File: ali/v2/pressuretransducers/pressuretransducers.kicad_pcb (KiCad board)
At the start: 4 copper layers, 85 x 76 mm, 235 parts, among them J1 Conn_02x01, J10 Conn_01x02, J11 Conn_01x02, J12 Conn_01x02, J13 Conn_01x02, J14 Conn_01x02, J15 Conn_01x02, J16 Conn_01x02, J17 Conn_01x02, J18 Conn_01x02, J19 Conn_01x02, J2 Conn_01x05, J20 Conn_01x02, J21 Conn_01x02, J22 Conn_01x02, J23 Conn_01x02, J24 Conn_01x02, J25 Conn_01x02, J3 USB_C_Receptacle_USB2.0_16P, J4 Conn_01x15, J5 Conn_02x09_Counter_Clockwise, J6 Screw_Terminal_01x02, J7 Screw_Terminal_01x02, J8 Conn_01x03, J9 Vertical Ethernet, SW1 SKRPANE010, U1 STM32H563RIV6, U2 AP2112K-3.3, U3 TJA1462ATK, U4 LAN8742AI, U5 ADS131M08IRSN, U6 ADS131M08IRSN, Y1 25 MHz, Y2 8.192 MHz, Y3 25 MHz

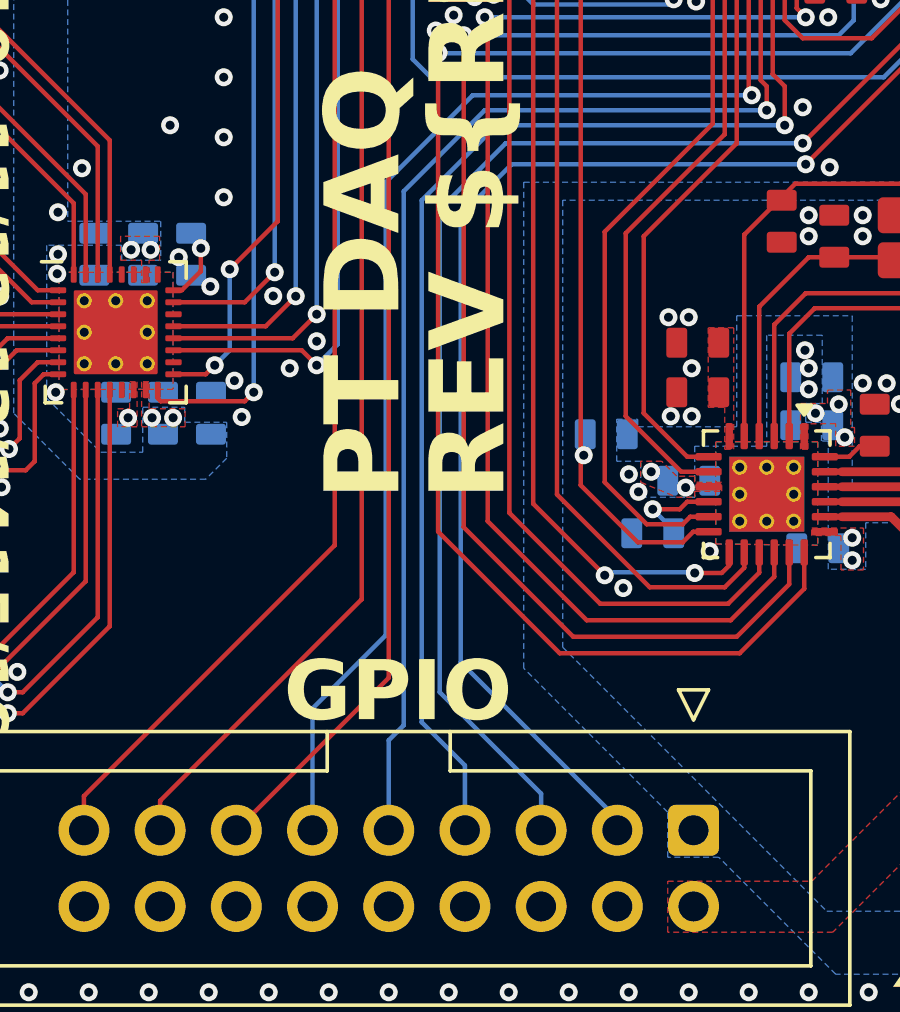
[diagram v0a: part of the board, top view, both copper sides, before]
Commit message: Minor thermocouple updates
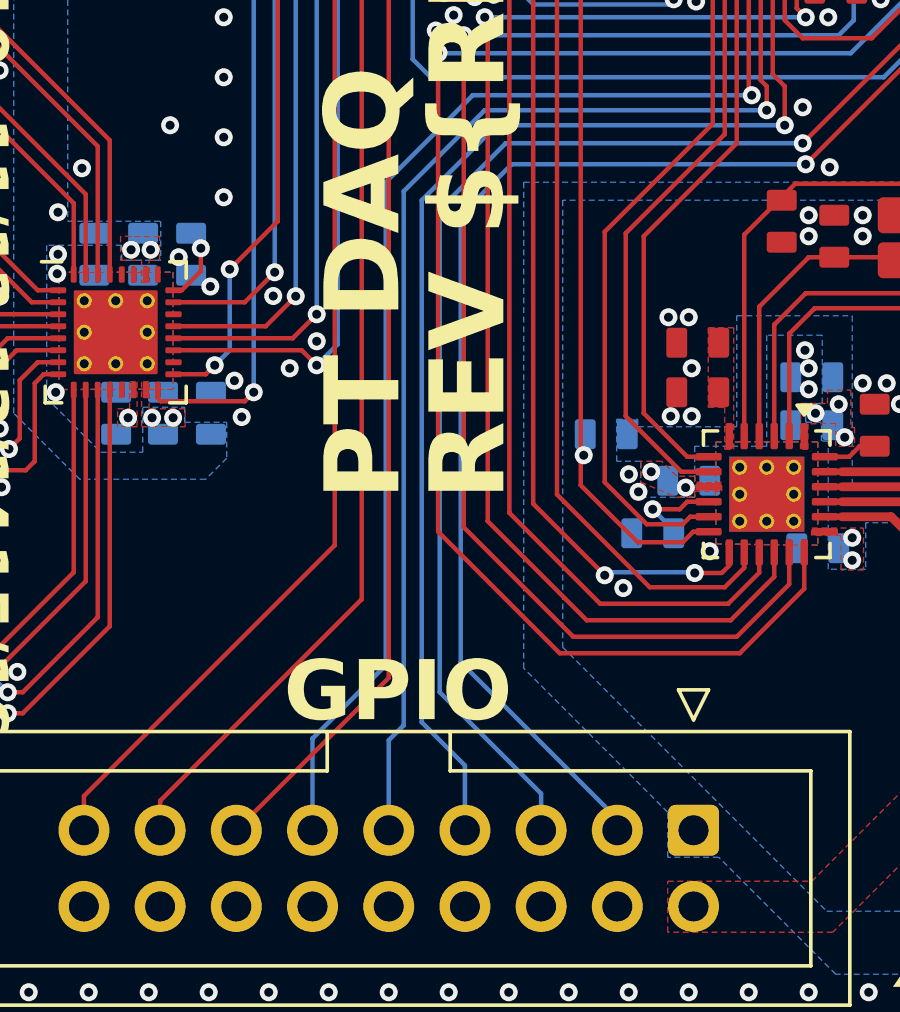
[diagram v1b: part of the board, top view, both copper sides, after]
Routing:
- net /Connectivity/ETH_MDIO: track 26.1 -> 26.8 mm
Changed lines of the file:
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@@
+	)
+	(segment
+		(start 140.2625 120.375)
+		(end 140.2125 120.425)
+		(width 0.3)
+		(layer "B.Cu")
+		(net "/Connectivity/ETH_MDIO")
+	)
+	(segment
+		(start 140.2625 119.725)
+		(end 140.2625 120.375)
+		(width 0.3)
+		(layer "B.Cu")
+		(net "/Connectivity/ETH_MDIO")
 	)
 	(segment
@@
 	)
 	(segment
+		(start 131.1725 129.865)
+		(end 131.1725 132.925)
+		(width 0.15)
+		(layer "B.Cu")
+		(net "/Microcontroller/PB0")
+	)
+	(segment
+		(start 136.5125 108.425)
+		(end 133.6125 111.325)
+		(width 0.15)
+		(layer "B.Cu")
+		(net "/Microcontroller/PB0")
+	)
+	(segment
 		(start 145.8125 108.425)
 		(end 136.5125 108.425)
@@
 	)
 	(segment
-		(start 131.1725 128.865)
-		(end 131.1725 132.925)
-		(width 0.15)
-		(layer "B.Cu")
-		(net "/Microcontroller/PB0")
-	)
-	(segment
-		(start 133.6125 126.425)
-		(end 131.1725 128.865)
-		(width 0.15)
-		(layer "B.Cu")
-		(net "/Microcontroller/PB0")
-	)
-	(segment
-		(start 136.5125 108.425)
-		(end 133.6125 111.325)
+		(start 133.6125 127.425)
+		(end 131.1725 129.865)
 		(width 0.15)
 		(layer "B.Cu")
@@
 	(segment
 		(start 133.6125 111.325)
-		(end 133.6125 126.425)
-		(width 0.15)
-		(layer "B.Cu")
+		(end 133.6125 127.425)
+		(width 0.15)
+		(layer "B.Cu")
